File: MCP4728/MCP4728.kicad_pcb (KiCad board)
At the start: 2 copper layers, 25.4 x 17.8 mm, 22 parts, among them J1 Conn_01x06, J2 Conn_01x04, J3 Conn_01x06, J4 Conn_01x04, U1 MCP4728

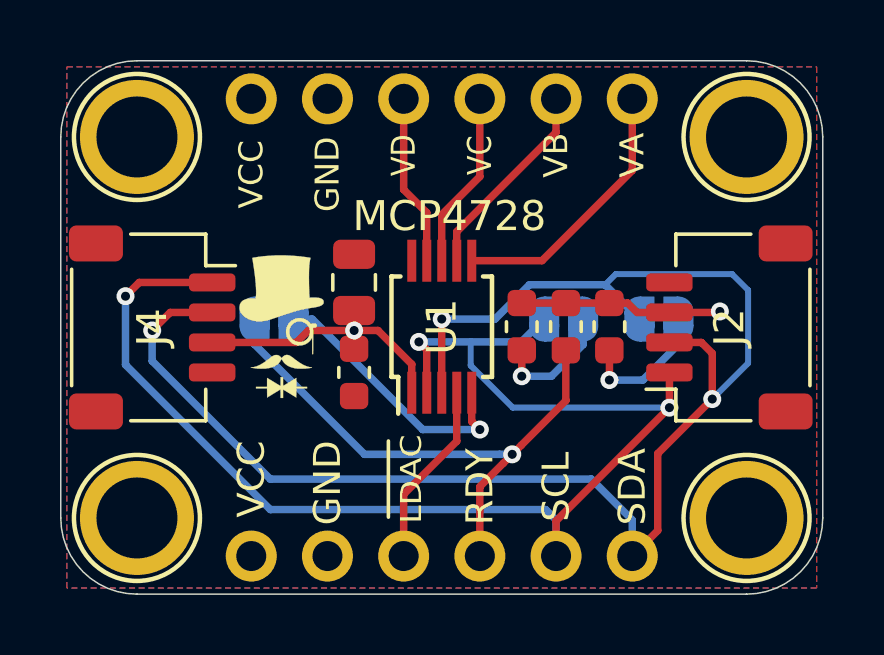
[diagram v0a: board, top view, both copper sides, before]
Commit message: Auto stash before revert of "Board Revision"
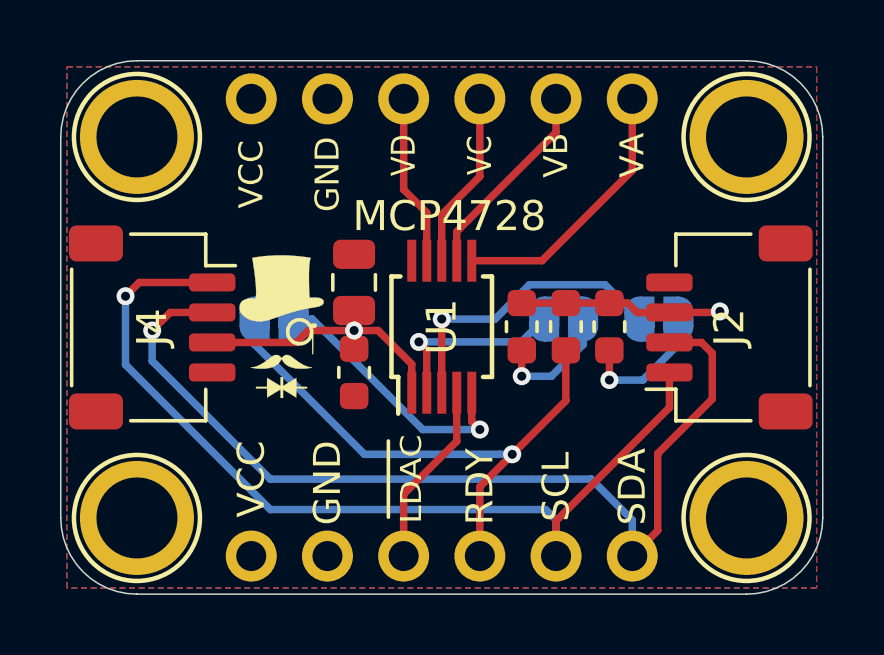
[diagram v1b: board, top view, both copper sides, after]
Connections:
- SCL pad 1: SCL_5V -> SCL
- SDA pad 1: SDA_5V -> SDA
- U1 pad 2: SCL_5V -> SCL
- U1 pad 3: SDA_5V -> SDA
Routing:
- net SDA_5V: track 51.4 -> 32.1 mm, vias 3 -> 1
- net SCL_5V: track 45.0 -> 30.7 mm, vias 3 -> 1
- net SDA: track 0.00 -> 9.99 mm, vias 0 -> 1
- net SCL: track 0.00 -> 6.29 mm, vias 0 -> 1
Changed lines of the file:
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@@
     (thickness 1.6)
     (drawings 32)
-    (tracks 108)
+    (tracks 95)
     (zones 0)
     (modules 22)
-    (nets 14)
+    (nets 16)
   )
   (page User 132.004 102.006)
   (title_block
     (title "MCP4728 Breakout")
-    (date 2020-03-10)
-    (rev 3)
+    (date 2020-01-23)
+    (rev 2)
     (company SirBoard)
     (comment 1 "4 Channel I2C DAC with 12 Bit Resolution")
@@
     (34 B.Paste user hide)
     (35 F.Paste user hide)
-    (36 B.SilkS user)
+    (36 B.SilkS user hide)
     (37 F.SilkS user)
     (38 B.Mask user hide)
@@
   )
   (setup
-    (last_trace_width 0.2)
+    (last_trace_width 0.127)
     (user_trace_width 0.2)
     (user_trace_width 0.25)
@@
   (net 11 "Net-(JP1-Pad2)")
   (net 12 "Net-(JP2-Pad2)")
-  (net 13 "Net-(JP3-Pad2)")
+  (net 13 SCL)
+  (net 14 "Net-(JP3-Pad2)")
+  (net 15 SDA)
   (net_class Default "This is the default net class."
     (clearance 0.127)
@@
     (add_net "Net-(JP3-Pad2)")
     (add_net RDY)
+    (add_net SCL)
     (add_net SCL_5V)
+    (add_net SDA)
     (add_net SDA_5V)
     (add_net VCC)
@@
       (net 6 LDAC))
     (pad 3 smd rect (at -2.2 0 90) (size 1.4 0.3) (layers F.Cu F.Paste F.Mask)
-      (net 3 SDA_5V))
+      (net 15 SDA))
     (pad 2 smd rect (at -2.2 -0.5 90) (size 1.4 0.3) (layers F.Cu F.Paste F.Mask)
-      (net 2 SCL_5V))
+      (net 13 SCL))
     (pad 1 smd rect (at -2.2 -1 90) (size 1.4 0.3) (layers F.Cu F.Paste F.Mask)
       (net 4 VCC))
@@
     (fp_line (start -0.8 0.4) (end -0.8 -0.4) (layer F.Fab) (width 0.1))
     (pad 2 smd roundrect (at 0.7875 0 270) (size 0.875 0.95) (layers F.Cu F.Paste F.Mask) (roundrect_rratio 0.25)
-      (net 13 "Net-(JP3-Pad2)"))
+      (net 14 "Net-(JP3-Pad2)"))
     (pad 1 smd roundrect (at -0.7875 0 270) (size 0.875 0.95) (layers F.Cu F.Paste F.Mask) (roundrect_rratio 0.25)
       (net 4 VCC))
@@
     (fp_arc (start 0.7 0.3) (end 1.4 0.3) (angle 90) (layer B.SilkS) (width 0.12))
     (pad 2 smd custom (at 0.65 0) (size 1 0.5) (layers B.Cu B.Mask)
-      (net 13 "Net-(JP3-Pad2)") (zone_connect 2)
+      (net 14 "Net-(JP3-Pad2)") (zone_connect 2)
       (options (clearance outline) (anchor rect))
       (primitives
@@
       ))
     (pad 1 smd custom (at -0.65 0) (size 1 0.5) (layers B.Cu B.Mask)
-      (net 3 SDA_5V) (zone_connect 2)
+      (net 15 SDA) (zone_connect 2)
       (options (clearance outline) (anchor rect))
       (primitives
@@
       ))
     (pad 1 smd custom (at -0.65 0) (size 1 0.5) (layers B.Cu B.Mask)
-      (net 2 SCL_5V) (zone_connect 2)
+      (net 13 SCL) (zone_connect 2)
       (options (clearance outline) (anchor rect))
       (primitives
@@
   (segment (start 69.992 36.534592) (end 68.934592 37.592) (width 0.25) (layer B.Cu) (net 12))
   (segment (start 67.945 37.592) (end 67.945 36.7285) (width 0.25) (layer F.Cu) (net 12))
-  (segment (start 64.778 36.711) (end 64.516 36.449) (width 0.25) (layer F.Cu) (net 2))
-  (segment (start 64.778 38.141) (end 64.778 36.711) (width 0.25) (layer F.Cu) (net 2))
-  (via (at 64.516 36.449) (size 0.6) (drill 0.3) (layers F.Cu B.Cu) (net 2))
-  (segment (start 68.692 35.687) (end 67.93 36.449) (width 0.25) (layer B.Cu) (net 2))
-  (segment (start 72.8665 38.6395) (end 72.8665 38.6395) (width 0.25) (layer F.Cu) (net 2))
-  (via (at 72.8665 38.6395) (size 0.6) (drill 0.3) (layers F.Cu B.Cu) (net 2))
-  (segment (start 66.2432 36.449) (end 66.2432 37.2364) (width 0.2) (layer B.Cu) (net 2))
-  (segment (start 67.93 36.449) (end 66.2432 36.449) (width 0.25) (layer B.Cu) (net 2))
-  (segment (start 66.2432 36.449) (end 64.516 36.449) (width 0.25) (layer B.Cu) (net 2))
-  (segment (start 67.6463 38.6395) (end 72.8665 38.6395) (width 0.2) (layer B.Cu) (net 2))
-  (segment (start 66.2432 37.2364) (end 67.6463 38.6395) (width 0.2) (layer B.Cu) (net 2))
-  (via (at 70.866 37.719) (size 0.6) (drill 0.3) (layers F.Cu B.Cu) (net 13))
-  (segment (start 71.982592 37.719) (end 70.866 37.719) (width 0.25) (layer B.Cu) (net 13))
-  (segment (start 73.167 35.687) (end 73.167 36.534592) (width 0.25) (layer B.Cu) (net 13))
-  (segment (start 73.167 36.534592) (end 71.982592 37.719) (width 0.25) (layer B.Cu) (net 13))
-  (segment (start 70.866 37.719) (end 70.866 36.7285) (width 0.25) (layer F.Cu) (net 13))
-  (segment (start 71.867 35.687) (end 70.724 34.544) (width 0.25) (layer B.Cu) (net 3))
-  (segment (start 70.724 34.544) (end 68.199 34.544) (width 0.25) (layer B.Cu) (net 3))
-  (via (at 65.278 35.687) (size 0.6) (drill 0.3) (layers F.Cu B.Cu) (net 3))
-  (segment (start 68.199 34.544) (end 67.056 35.687) (width 0.25) (layer B.Cu) (net 3))
-  (segment (start 67.056 35.687) (end 65.278 35.687) (width 0.25) (layer B.Cu) (net 3))
-  (segment (start 65.278 35.687) (end 65.278 38.141) (width 0.25) (layer F.Cu) (net 3))
-  (segment (start 74.295 38.354) (end 74.295 38.354) (width 0.25) (layer F.Cu) (net 3))
-  (via (at 74.295 38.354) (size 0.6) (drill 0.3) (layers F.Cu B.Cu) (net 3))
-  (segment (start 70.724 34.544) (end 71.0796 34.1884) (width 0.2) (layer B.Cu) (net 3))
-  (segment (start 71.0796 34.1884) (end 74.9554 34.1884) (width 0.2) (layer B.Cu) (net 3))
-  (segment (start 74.9554 34.1884) (end 75.4888 34.7218) (width 0.2) (layer B.Cu) (net 3))
-  (segment (start 75.4888 37.1602) (end 74.295 38.354) (width 0.2) (layer B.Cu) (net 3))
-  (segment (start 75.4888 34.7218) (end 75.4888 37.1602) (width 0.2) (layer B.Cu) (net 3))
+  (segment (start 64.778 36.711) (end 64.516 36.449) (width 0.25) (layer F.Cu) (net 13))
+  (segment (start 64.778 38.141) (end 64.778 36.711) (width 0.25) (layer F.Cu) (net 13))
+  (via (at 64.516 36.449) (size 0.6) (drill 0.3) (layers F.Cu B.Cu) (net 13))
+  (segment (start 67.93 36.449) (end 64.516 36.449) (width 0.25) (layer B.Cu) (net 13))
+  (segment (start 68.692 35.687) (end 67.93 36.449) (width 0.25) (layer B.Cu) (net 13))
+  (via (at 70.866 37.719) (size 0.6) (drill 0.3) (layers F.Cu B.Cu) (net 14))
+  (segment (start 71.982592 37.719) (end 70.866 37.719) (width 0.25) (layer B.Cu) (net 14))
+  (segment (start 73.167 35.687) (end 73.167 36.534592) (width 0.25) (layer B.Cu) (net 14))
+  (segment (start 73.167 36.534592) (end 71.982592 37.719) (width 0.25) (layer B.Cu) (net 14))
+  (segment (start 70.866 37.719) (end 70.866 36.7285) (width 0.25) (layer F.Cu) (net 14))
+  (segment (start 71.867 35.687) (end 70.724 34.544) (width 0.25) (layer B.Cu) (net 15))
+  (segment (start 70.724 34.544) (end 68.199 34.544) (width 0.25) (layer B.Cu) (net 15))
+  (via (at 65.278 35.687) (size 0.6) (drill 0.3) (layers F.Cu B.Cu) (net 15))
+  (segment (start 68.199 34.544) (end 67.056 35.687) (width 0.25) (layer B.Cu) (net 15))
+  (segment (start 67.056 35.687) (end 65.278 35.687) (width 0.25) (layer B.Cu) (net 15))
+  (segment (start 65.278 35.687) (end 65.278 38.141) (width 0.25) (layer F.Cu) (net 15))
   (zone (net 4) (net_name VCC) (layer B.Cu) (hatch none 0.508)
     (connect_pads (clearance 0.15))
